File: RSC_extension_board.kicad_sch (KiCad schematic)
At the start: 23 parts, among them J1 Conn_01x03, J2 Conn_01x03, J3 Conn_01x03, J4 Raspberry_Pi_4, J5 Conn_01x04, J6 USB_C_Receptacle_PowerOnly_6P, J7 Conn_01x02, Q1 BSS138, U1 USBLC6-2SC6

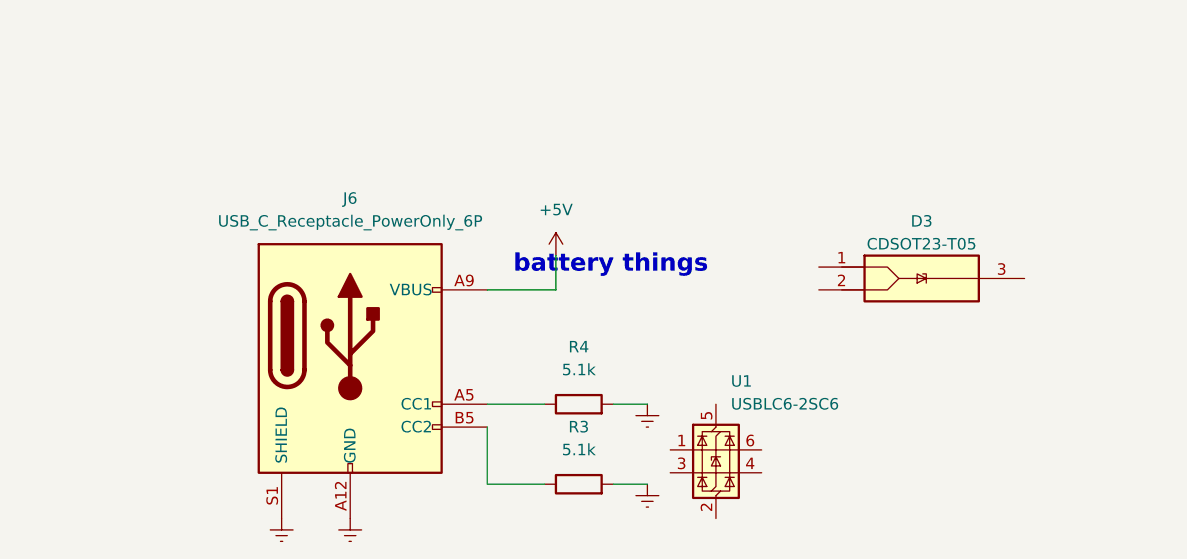
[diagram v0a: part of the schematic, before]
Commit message: some external power stuff
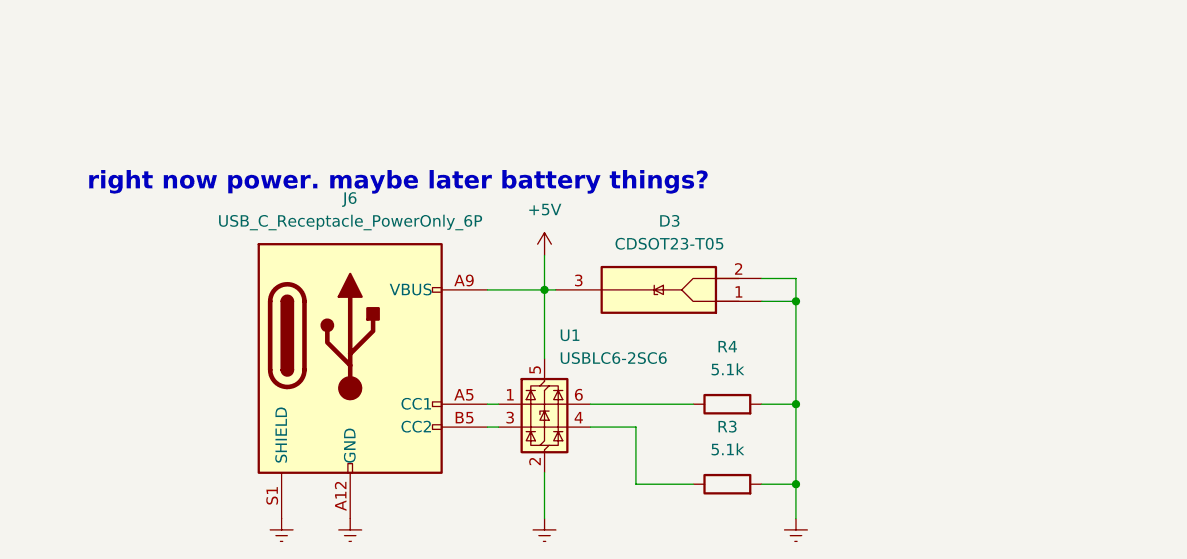
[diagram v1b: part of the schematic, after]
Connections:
- net +5V: now also D3.3, U1.5 (VBUS)
- net Earth: now also D3.1, D3.2, U1.2 (GND)
- net at R3.1: now also U1.4 (I/O2); no longer J6.B5 (CC2)
- net at R4.1: now also U1.6 (I/O1); no longer J6.A5 (CC1)
- net at U1.1 (I/O1): now also J6.A5 (CC1)
- net at U1.3 (I/O2): now also J6.B5 (CC2)
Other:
- note added: "right now power. maybe later battery things?"
- note removed: "battery things"
- moved on the sheet: D3, R3, R4, U1
